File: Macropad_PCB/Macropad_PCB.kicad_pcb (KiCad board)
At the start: 2 copper layers, 91 x 85.5 mm, 27 parts, among them J1 OLED_128x32, SW0 RotaryEncoder, U1 MOUDLE-SEEEDUINO-XIAO

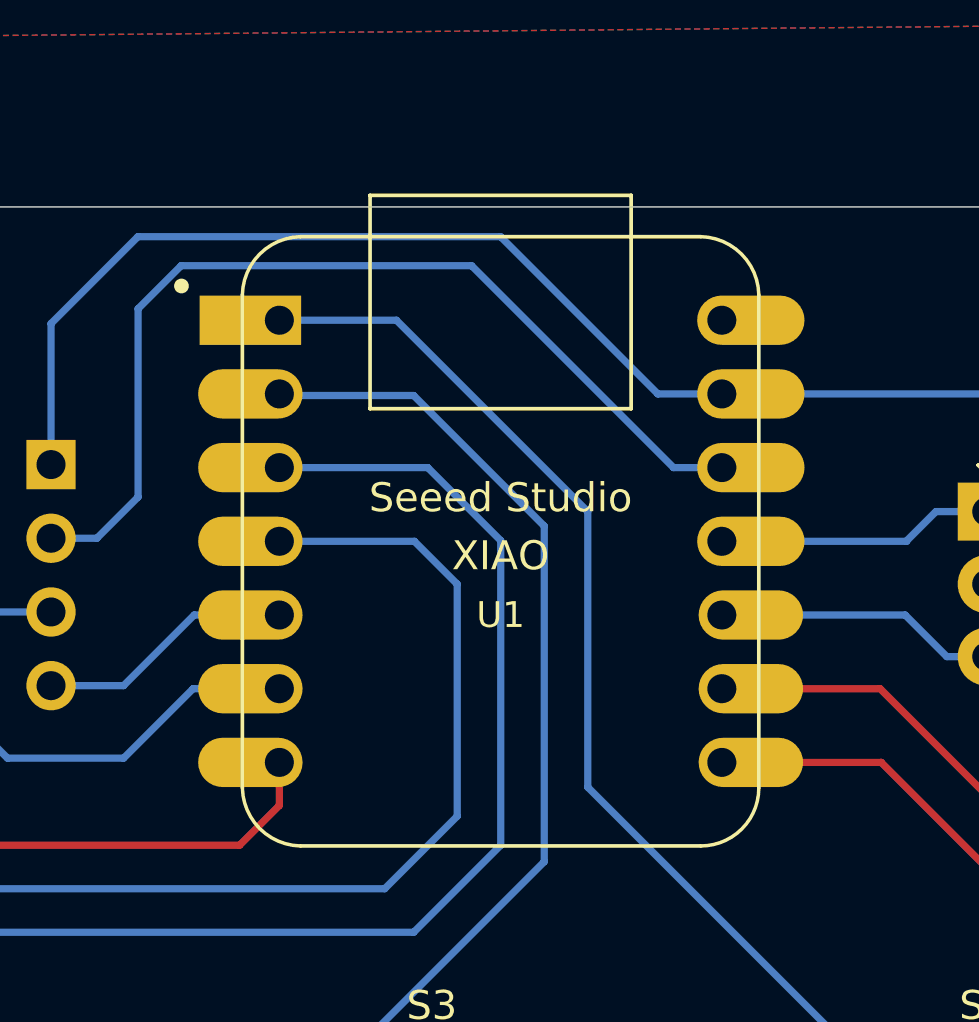
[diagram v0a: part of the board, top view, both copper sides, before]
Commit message: PCB finito (in teoria)
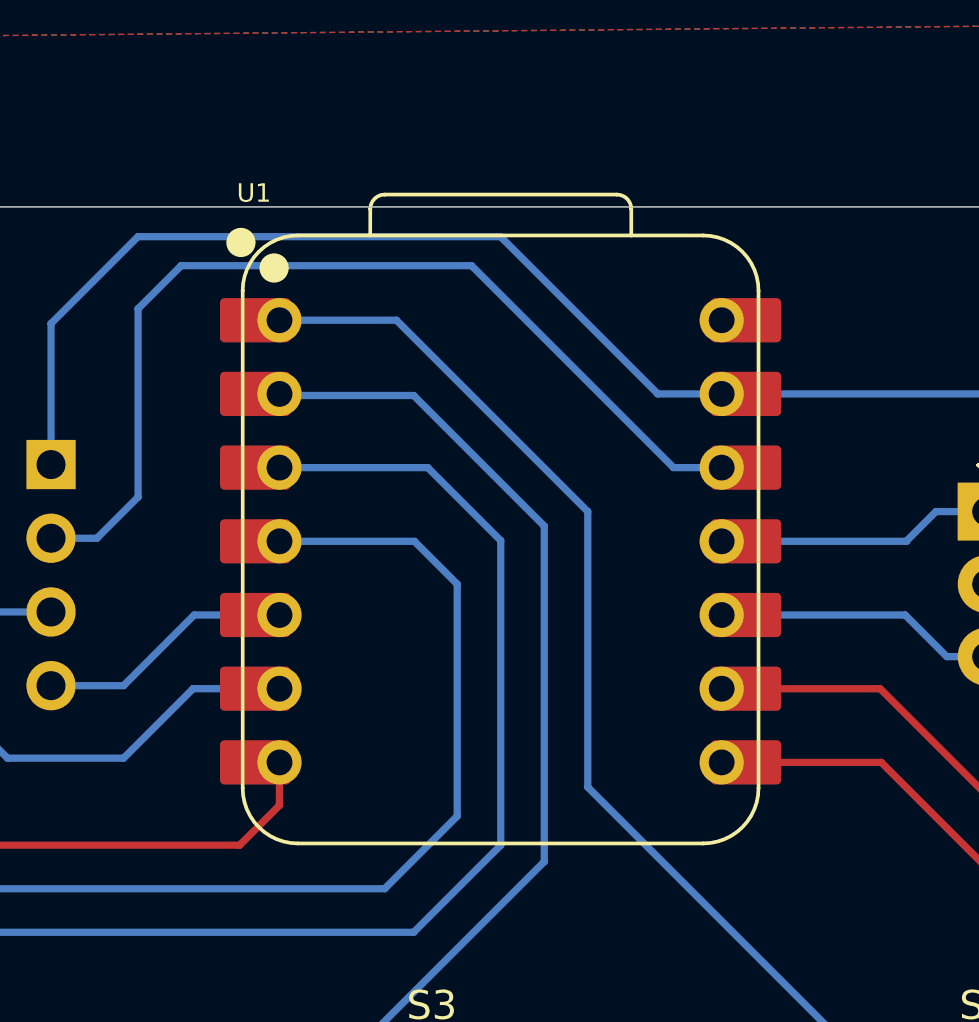
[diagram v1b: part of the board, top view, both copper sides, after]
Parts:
- U1: footprint footprints:XIAO-Generic-Hybrid-14P-2.54-21X17.8MM -> Seeed Studio XIAO Series Library:XIAO-RP2040-DIP
